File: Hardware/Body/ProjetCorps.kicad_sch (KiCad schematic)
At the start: 38 parts, among them J1 Conn_01x04, J101 Conn_01x02, J102 Conn_01x03, J103 Conn_01x03, J104 Conn_01x15, J105 Conn_ST_STDC14, J2 Conn_01x06, J3 Conn_01x04, SW1 SW_SPST, SW101 SW_SPDT, U1 STM32G474RETx, U103 AZ1117-3.3, U104 173010542

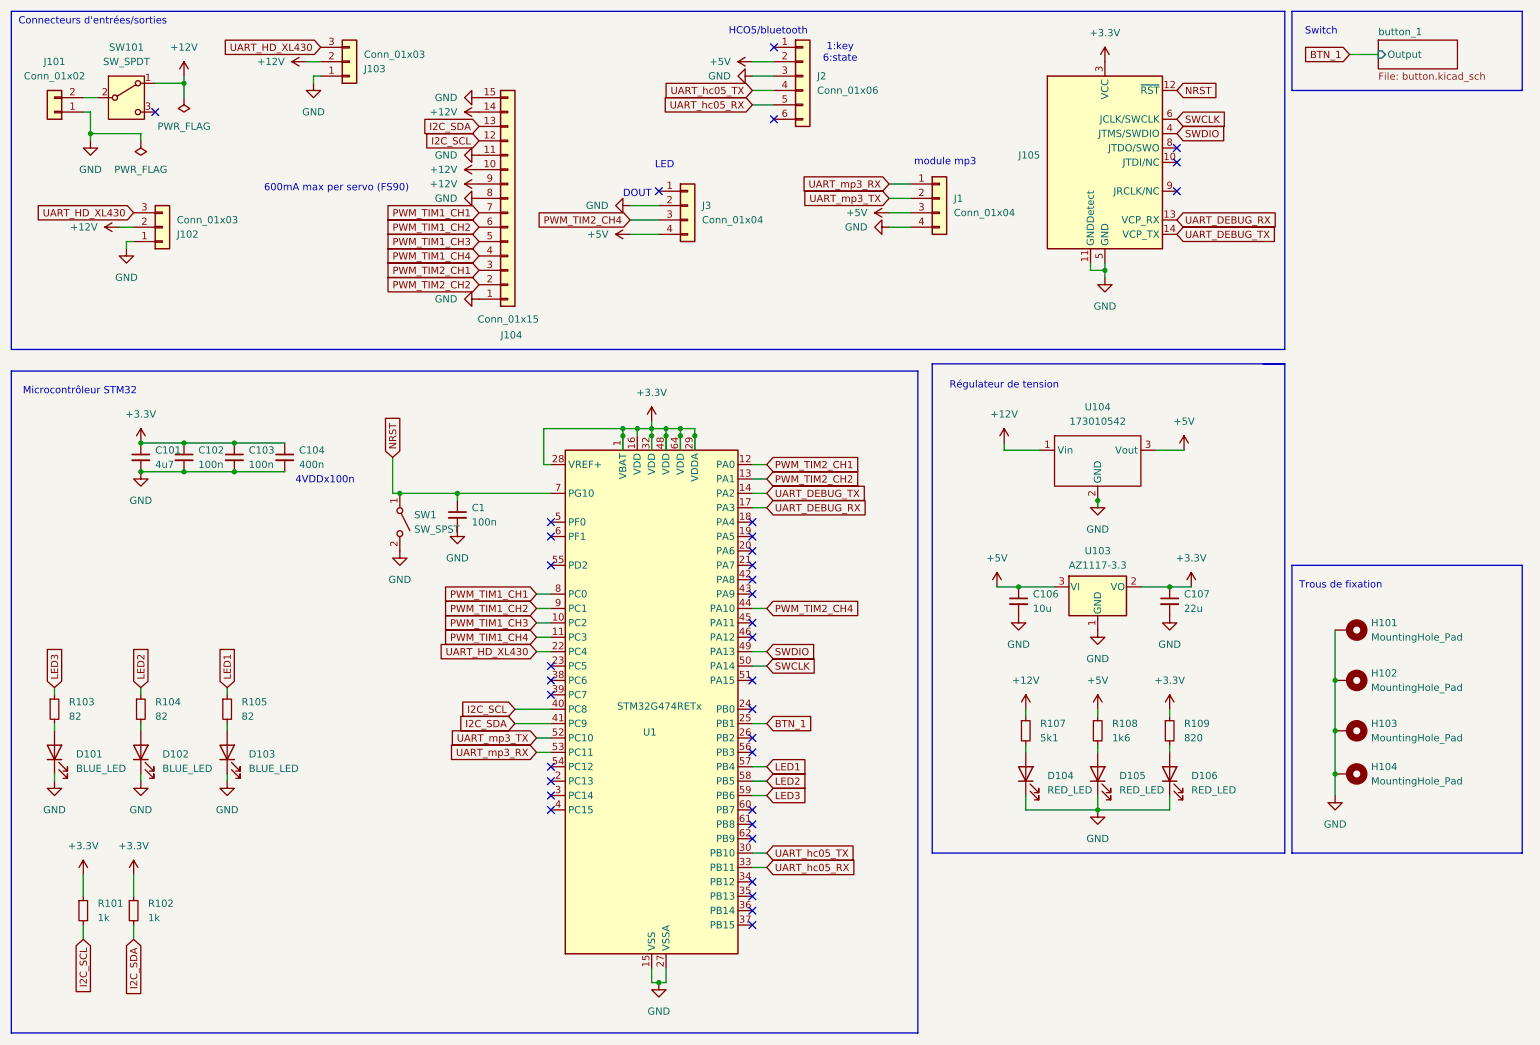
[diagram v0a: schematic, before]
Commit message: check Fiack
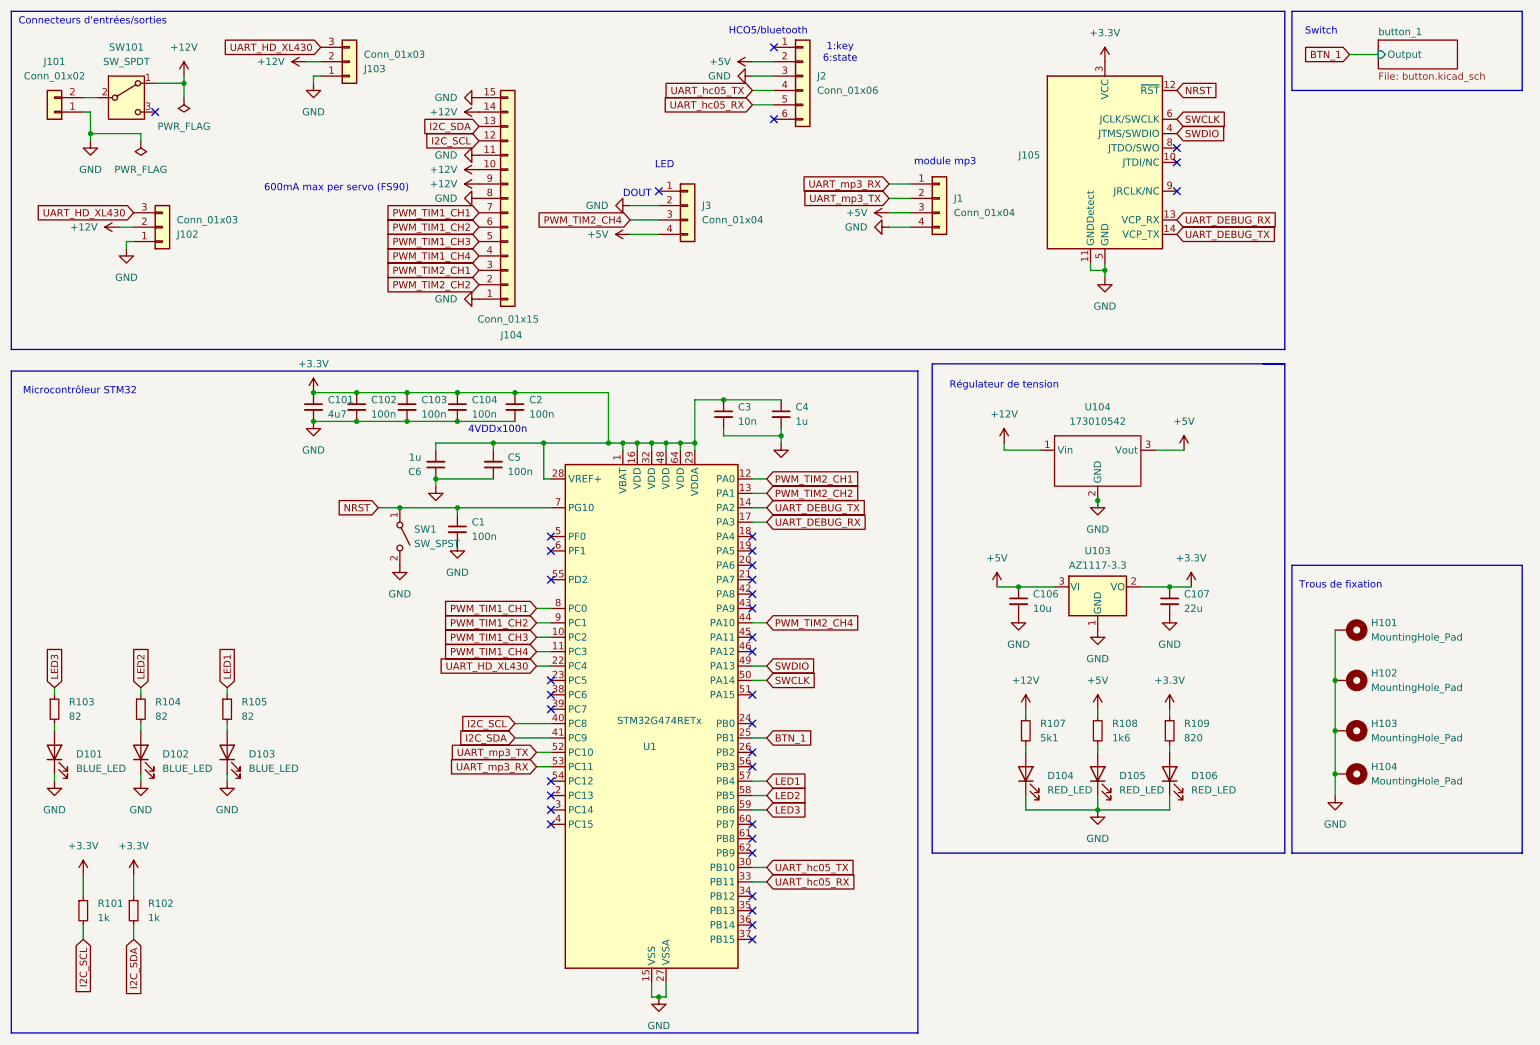
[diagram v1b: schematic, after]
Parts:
- added C2, C5: 100n, Capacitor_SMD:C_0402_1005Metric, symbol Device:C_Small
- added C3: 10n, Capacitor_SMD:C_0402_1005Metric, symbol Device:C_Small
- added C4, C6: 1u, Capacitor_SMD:C_0402_1005Metric, symbol Device:C_Small
- C104: value 400n -> 100n
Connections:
- net +3.3V: now also C2.1, C3.1, C4.1, C5.2, C6.2
- net GND: now also C2.2, C3.2, C4.2, C5.1, C6.1
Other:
- moved on the sheet: C1, C101, C102, C103, C104, SW1, U1
